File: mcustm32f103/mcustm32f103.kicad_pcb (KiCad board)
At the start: 2 copper layers, 76.2 x 50.8 mm, 31 parts, among them J2 STM32WORLD_BASE, U1 AMS1117-3.3, U2 STM32F405RGTx, U3 SRV05-4, Y1 X_16MHZ

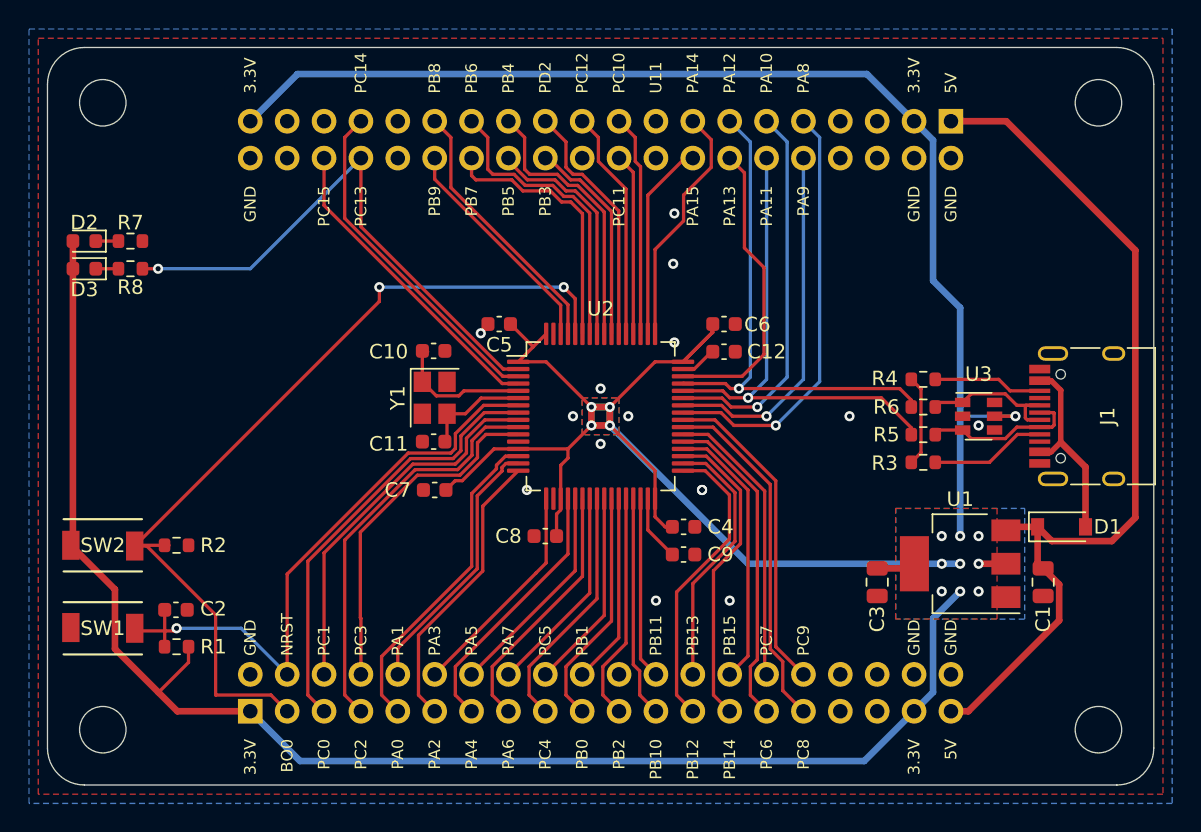
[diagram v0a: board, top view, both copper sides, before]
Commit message: Hmmm
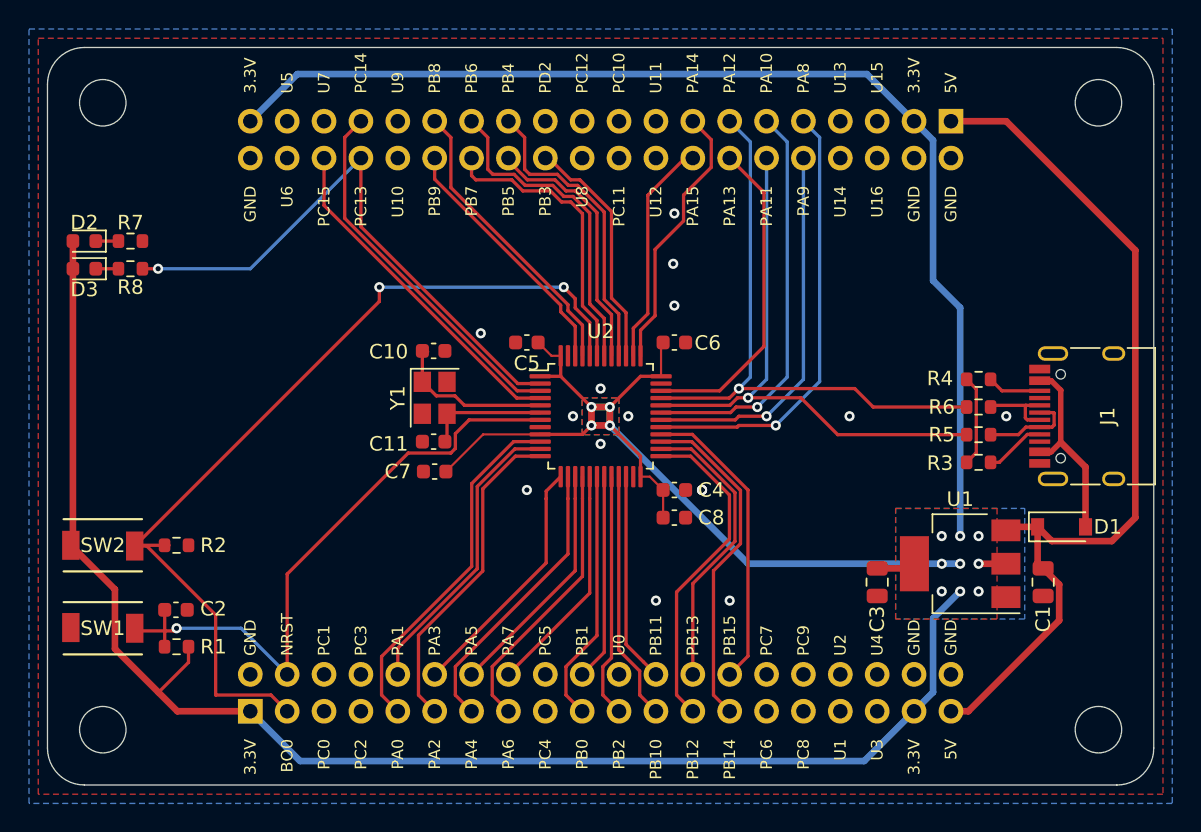
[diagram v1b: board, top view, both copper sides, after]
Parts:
- removed C12, C9: C_2.2UF_0603, Capacitor_SMD:C_0603_1608Metric
- removed U3: SRV05-4, Package_TO_SOT_SMD:SOT-23-6
- U2: value STM32F405RGTx -> STM32F103CBTx; footprint Package_QFP:LQFP-64_10x10mm_P0.5mm -> Package_QFP:LQFP-48_7x7mm_P0.5mm
- moved C8 8.98 mm to (157.5, 108.6), turned to 0 degrees
- moved R3 3.81 mm to (178.4, 104.8)
- moved R4 3.81 mm to (178.4, 99.1)
- moved R5 3.81 mm to (178.4, 102.9)
- moved R6 3.81 mm to (178.4, 101.0)
- moved C6 3.65 mm to (157.5, 96.5)
- moved C4 2.62 mm to (157.5, 106.7)
- moved C5 2.29 mm to (147.3, 96.5)
- moved C7 1.27 mm to (141.0, 105.4)
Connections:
- U2 pad 10: PC2 -> PA0
- U2 pad 11: PC3 -> PA1
- U2 pad 12: GND -> PA2
- U2 pad 13: +3V3 -> PA3
- U2 pad 14: PA0 -> PA4
- U2 pad 15: PA1 -> PA5
- U2 pad 16: PA2 -> PA6
- U2 pad 17: PA3 -> PA7
- U2 pad 18: GND -> PB0
- U2 pad 19: +3V3 -> PB1
- U2 pad 20: PA4 -> PB2
- U2 pad 21: PA5 -> PB10
- U2 pad 22: PA6 -> PB11
- U2 pad 23: PA7 -> GND
- U2 pad 24: PC4 -> +3V3
- U2 pad 25: PC5 -> PB12
- U2 pad 26: PB0 -> PB13
- U2 pad 27: PB1 -> PB14
- U2 pad 28: PB2 -> PB15
- U2 pad 29: PB10 -> PA8
- U2 pad 30: PB11 -> PA9
- U2 pad 31: Net-(C9-Pad1) -> PA10
- U2 pad 32: +3V3 -> PA11
- U2 pad 33: PB12 -> PA12
- U2 pad 34: PB13 -> PA13
- U2 pad 35: PB14 -> GND
- U2 pad 36: PB15 -> +3V3
- U2 pad 37: PC6 -> PA14
- U2 pad 38: PC7 -> PA15
- U2 pad 39: PC8 -> PB3
- U2 pad 40: PC9 -> PB4
- U2 pad 41: PA8 -> PB5
- U2 pad 42: PA9 -> PB6
- U2 pad 43: PA10 -> PB7
- U2 pad 44: PA11 -> BO0
- U2 pad 45: PA12 -> PB8
- U2 pad 46: PA13 -> PB9
- U2 pad 47: Net-(C12-Pad1) -> GND
- U2 pad 8: PC0 -> GND
- U2 pad 9: PC1 -> +3V3
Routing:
- net PC0: track 30.1 -> 0.00 mm
- net PC2: track 28.0 -> 0.00 mm
- net PC1: track 26.1 -> 0.00 mm
- net PC8: track 24.2 -> 0.00 mm
- net PC3: track 24.1 -> 0.00 mm
- net +3V3: track 280.8 -> 257.9 mm, vias 14 -> 13
- net PC6: track 22.3 -> 0.00 mm
- net PC9: track 22.3 -> 0.00 mm
- net PC7: track 19.9 -> 0.00 mm
- net PD2: track 17.1 -> 0.00 mm
- net PC4: track 17.0 -> 0.00 mm
- net PC12: track 15.9 -> 0.00 mm
- net PC10: track 15.3 -> 0.00 mm
- net PC5: track 13.8 -> 0.00 mm
- net PC11: track 12.5 -> 0.00 mm
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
